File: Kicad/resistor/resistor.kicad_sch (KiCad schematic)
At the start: 145 parts, among them K1 R

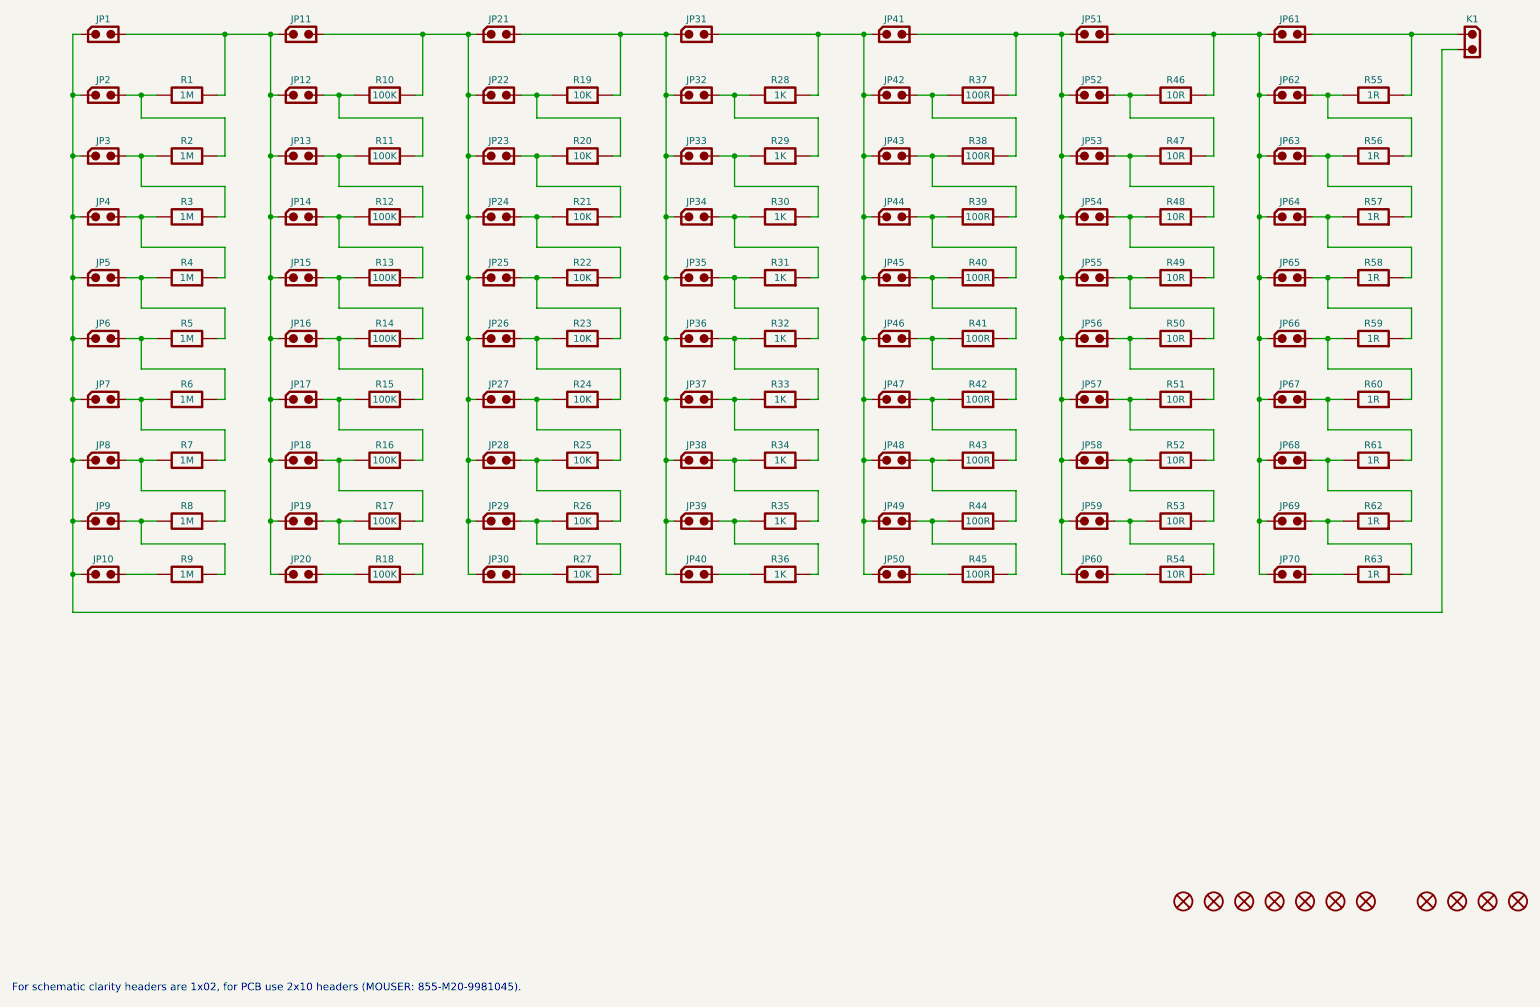
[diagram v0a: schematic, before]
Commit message: Up
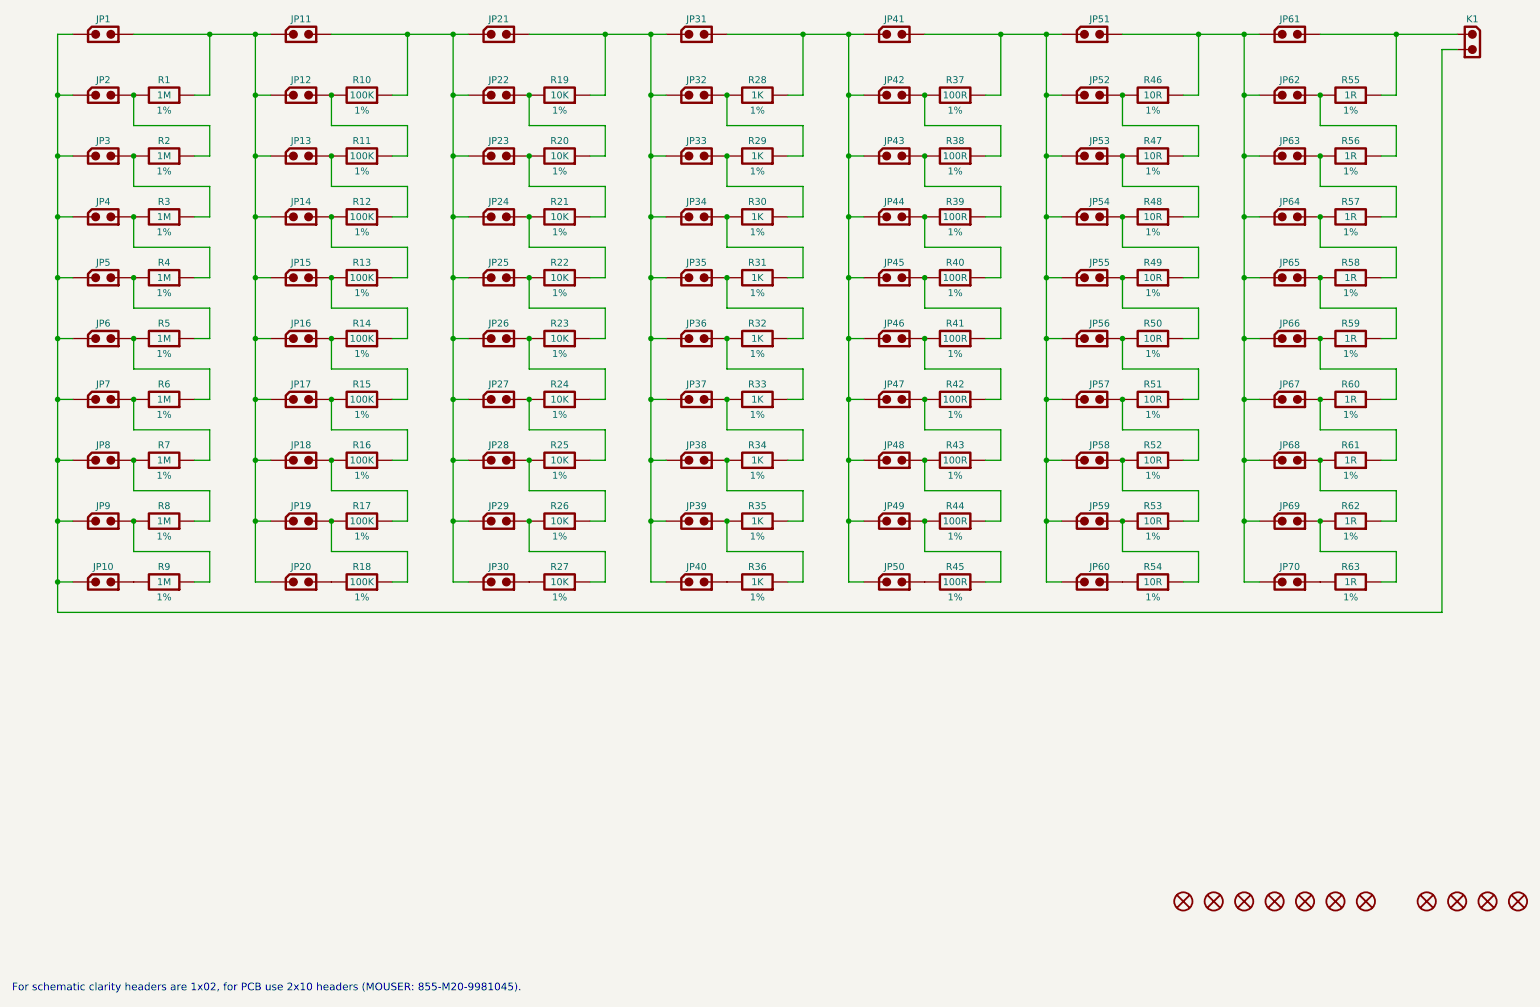
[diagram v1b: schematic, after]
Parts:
- JP1, JP10, JP11, JP12, JP13, JP14, JP15, JP16, JP17, JP18, JP19, JP2, JP20, JP21, JP22, JP23, JP24, JP25, JP26, JP27, JP28, JP29, JP3, JP30, JP31, JP32, JP33, JP34, JP35, JP36, JP37, JP38, JP39, JP4, JP40, JP41, JP42, JP43, JP44, JP45, JP46, JP47, JP48, JP49, JP5, JP50, JP51, JP52, JP53, JP54, JP55, JP56, JP57, JP58, JP59, JP6, JP60, JP61, JP62, JP63, JP64, JP65, JP66, JP67, JP68, JP69, JP7, JP70, JP8, JP9: Name HARWIN-254-M-1X02-JUMPER-VERTICAL -> (none)
- R1, R2, R3, R4, R5, R6, R7, R8, R9: Name RESISTOR-1206-1M-1P -> (none)
- R10, R11, R12, R13, R14, R15, R16, R17, R18: Name RESISTOR-1206-100K-1P -> (none)
- R19, R20, R21, R22, R23, R24, R25, R26, R27: Name RESISTOR-1206-10K-1P -> (none)
- R28, R29, R30, R31, R32, R33, R34, R35, R36: Mouser RT1206FRE071KL -> 603-RT1206FRE071KL; Name RESISTOR-1206-1K-1P -> (none)
- R37, R38, R39, R40, R41, R42, R43, R44, R45: Name RESISTOR-1206-100R-1P -> (none)
- R46, R47, R48, R49, R50, R51, R52, R53, R54: Name RESISTOR-1206-10R-1P -> (none)
- R55, R56, R57, R58, R59, R60, R61, R62, R63: Name RESISTOR-1206-1R-1P -> (none)
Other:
- moved on the sheet: JP10, JP20, JP30, JP40, JP50, JP60, JP70, R1, R10, R19, R28, R37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
